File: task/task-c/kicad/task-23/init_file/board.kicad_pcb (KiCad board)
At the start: 4 copper layers, 80 x 40 mm, 4 parts

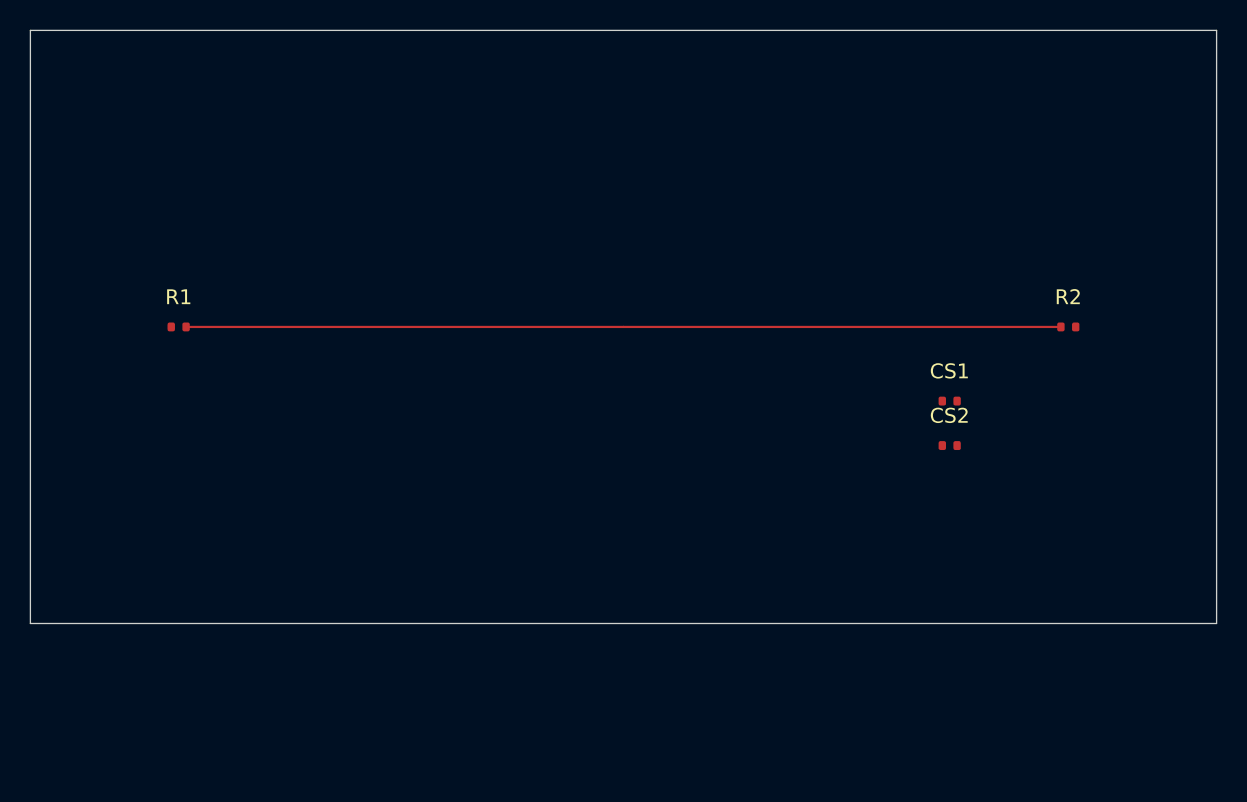
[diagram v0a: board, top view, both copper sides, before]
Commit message: Refine engineering task metadata and instructions
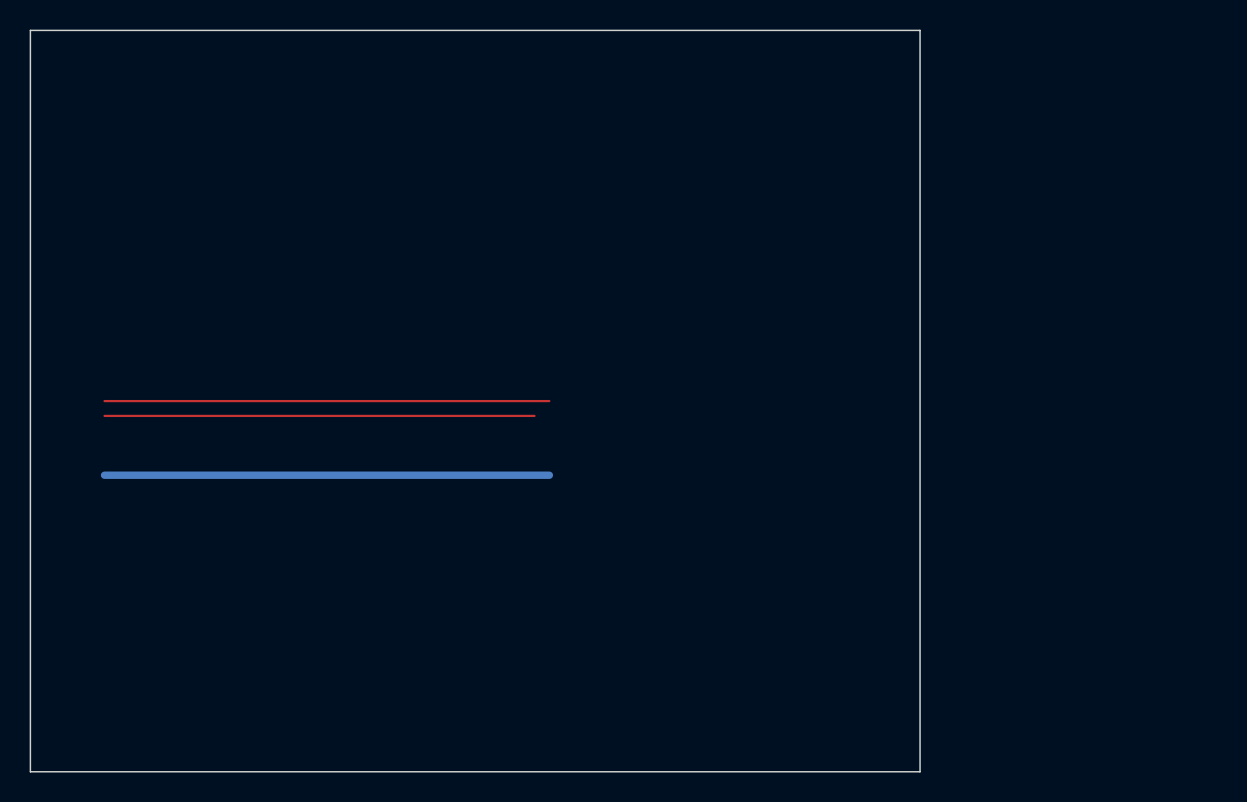
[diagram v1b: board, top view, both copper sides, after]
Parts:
- removed CS1, CS2: 100n, Capacitor_SMD:C_0402
- removed R1, R2: 100, Resistor_SMD:R_0402
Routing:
- net HS1: track 59.0 -> 0.00 mm
- net USB_DP: track 0.00 -> 30.0 mm
- net GND: track 0.00 -> 30.0 mm
- net USB_DM: track 0.00 -> 29.0 mm
- removed copper zone on In1.Cu, net +3V3
- removed copper zone on In1.Cu, net GND
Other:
- board size 80 x 40 mm -> 60 x 50 mm
- copper layers 4 -> 2
- rule pad_to_mask_clearance: 0.051 -> 0.1
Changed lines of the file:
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@@
   (version 20240108)
   (generator "pcbnew")
-  (general (thickness 1.6) (legacy_teardrops no))
+  (generator_version "9.0")
+  (general
+    (thickness 1.6)
+    (legacy_teardrops no)
+  )
   (paper "A4")
   (layers
     (0 "F.Cu" signal)
-    (1 "In1.Cu" power)
-    (2 "In2.Cu" power)
     (31 "B.Cu" signal)
-    (36 "B.SilkS" user "B.Silkscreen")
-    (37 "F.SilkS" user "F.Silkscreen")
-    (49 "Edge.Cuts" user)
+    (44 "Edge.Cuts" user)
   )
-  (setup (pad_to_mask_clearance 0.051))
+  (setup
+    (pad_to_mask_clearance 0.1)
+    (allow_soldermask_bridges_in_footprints no)
+  )
   (net 0 "")
-  (net 1 "GND")
-  (net 2 "+3V3")
-  (net 3 "HS1")
-  (net 4 "HS2")
-  (footprint "Resistor_SMD:R_0402"
-    (layer "F.Cu")
-    (at 10 20)
-    (property "Reference" "R1" (at 0 -2) (layer "F.SilkS") (effects (font (size 1 1) (thickness 0.15))))
-    (property "Value" "100" (at 0 2) (layer "F.Fab") (effects (font (size 1 1) (thickness 0.15))))
-    (pad "1" smd roundrect (at -0.5 0) (size 0.5 0.6) (layers "F.Cu" "F.Paste" "F.Mask") (roundrect_rratio 0.25) (net 3 "HS1"))
-    (pad "2" smd roundrect (at 0.5 0) (size 0.5 0.6) (layers "F.Cu" "F.Paste" "F.Mask") (roundrect_rratio 0.25) (net 3 "HS1"))
-  )
-  (footprint "Resistor_SMD:R_0402"
-    (layer "F.Cu")
-    (at 70 20)
-    (property "Reference" "R2" (at 0 -2) (layer "F.SilkS") (effects (font (size 1 1) (thickness 0.15))))
-    (property "Value" "100" (at 0 2) (layer "F.Fab") (effects (font (size 1 1) (thickness 0.15))))
-    (pad "1" smd roundrect (at -0.5 0) (size 0.5 0.6) (layers "F.Cu" "F.Paste" "F.Mask") (roundrect_rratio 0.25) (net 4 "HS2"))
-    (pad "2" smd roundrect (at 0.5 0) (size 0.5 0.6) (layers "F.Cu" "F.Paste" "F.Mask") (roundrect_rratio 0.25) (net 4 "HS2"))
-  )
-  (footprint "Capacitor_SMD:C_0402"
-    (layer "F.Cu")
-    (at 62 25)
-    (property "Reference" "CS1" (at 0 -2) (layer "F.SilkS") (effects (font (size 1 1) (thickness 0.15))))
-    (property "Value" "100n" (at 0 2) (layer "F.Fab") (effects (font (size 1 1) (thickness 0.15))))
-    (pad "1" smd roundrect (at -0.5 0) (size 0.5 0.6) (layers "F.Cu" "F.Paste" "F.Mask") (roundrect_rratio 0.25) (net 1 "GND"))
-    (pad "2" smd roundrect (at 0.5 0) (size 0.5 0.6) (layers "F.Cu" "F.Paste" "F.Mask") (roundrect_rratio 0.25) (net 2 "+3V3"))
-  )
-  (footprint "Capacitor_SMD:C_0402"
-    (layer "F.Cu")
-    (at 62 28)
-    (property "Reference" "CS2" (at 0 -2) (layer "F.SilkS") (effects (font (size 1 1) (thickness 0.15))))
-    (property "Value" "100n" (at 0 2) (layer "F.Fab") (effects (font (size 1 1) (thickness 0.15))))
-    (pad "1" smd roundrect (at -0.5 0) (size 0.5 0.6) (layers "F.Cu" "F.Paste" "F.Mask") (roundrect_rratio 0.25) (net 1 "GND"))
-    (pad "2" smd roundrect (at 0.5 0) (size 0.5 0.6) (layers "F.Cu" "F.Paste" "F.Mask") (roundrect_rratio 0.25) (net 2 "+3V3"))
-  )
-  (segment (start 10.5 20) (end 40 20) (width 0.15) (layer "F.Cu") (net 3))
-  (segment (start 40 20) (end 69.5 20) (width 0.15) (layer "F.Cu") (net 3))
-  (zone
-    (net 1)
-    (net_name "GND")
-    (layer "In1.Cu")
-    (name "GND_LEFT")
-    (hatch edge 0.508)
-    (connect_pads (clearance 0.25))
-    (min_thickness 0.25)
-    (fill yes (thermal_gap 0.5) (thermal_bridge_width 0.5))
-    (polygon (pts (xy 0 0) (xy 40 0) (xy 40 40) (xy 0 40)))
-  )
-  (zone
-    (net 2)
-    (net_name "+3V3")
-    (layer "In1.Cu")
-    (name "V33_RIGHT")
-    (hatch edge 0.508)
-    (connect_pads (clearance 0.25))
-    (min_thickness 0.25)
-    (fill yes (thermal_gap 0.5) (thermal_bridge_width 0.5))
-    (polygon (pts (xy 40 0) (xy 80 0) (xy 80 40) (xy 40 40)))
-  )
-  (gr_line (start 40 0) (end 40 40) (layer "Eco1.User") (width 0.1))
-  (gr_rect (start 0 0) (end 80 40) (layer "Edge.Cuts") (width 0.05))
+  (net 1 "USB_DP")
+  (net 2 "USB_DM")
+  (net 3 "GND")
+  (net 4 "VBUS")
+  (segment (start 5 25) (end 35 25) (width 0.15) (layer "F.Cu") (net 1))
+  (segment (start 5 26) (end 34 26) (width 0.15) (layer "F.Cu") (net 2))
+  (segment (start 5 30) (end 35 30) (width 0.5) (layer "B.Cu") (net 3))
+  (gr_rect (start 0 0) (end 60 50) (layer "Edge.Cuts") (width 0.1))
 )
